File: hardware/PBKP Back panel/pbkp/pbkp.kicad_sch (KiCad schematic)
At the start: 9 parts, among them J1 Mini-DIN-6, J2 Mini-DIN-6, J3 RCA, J4 DB25_Male, J5 DB25_Female, J5 DB9_Male, J6 DB9_Female, J7 DB25_Female, J8 DB9_Female

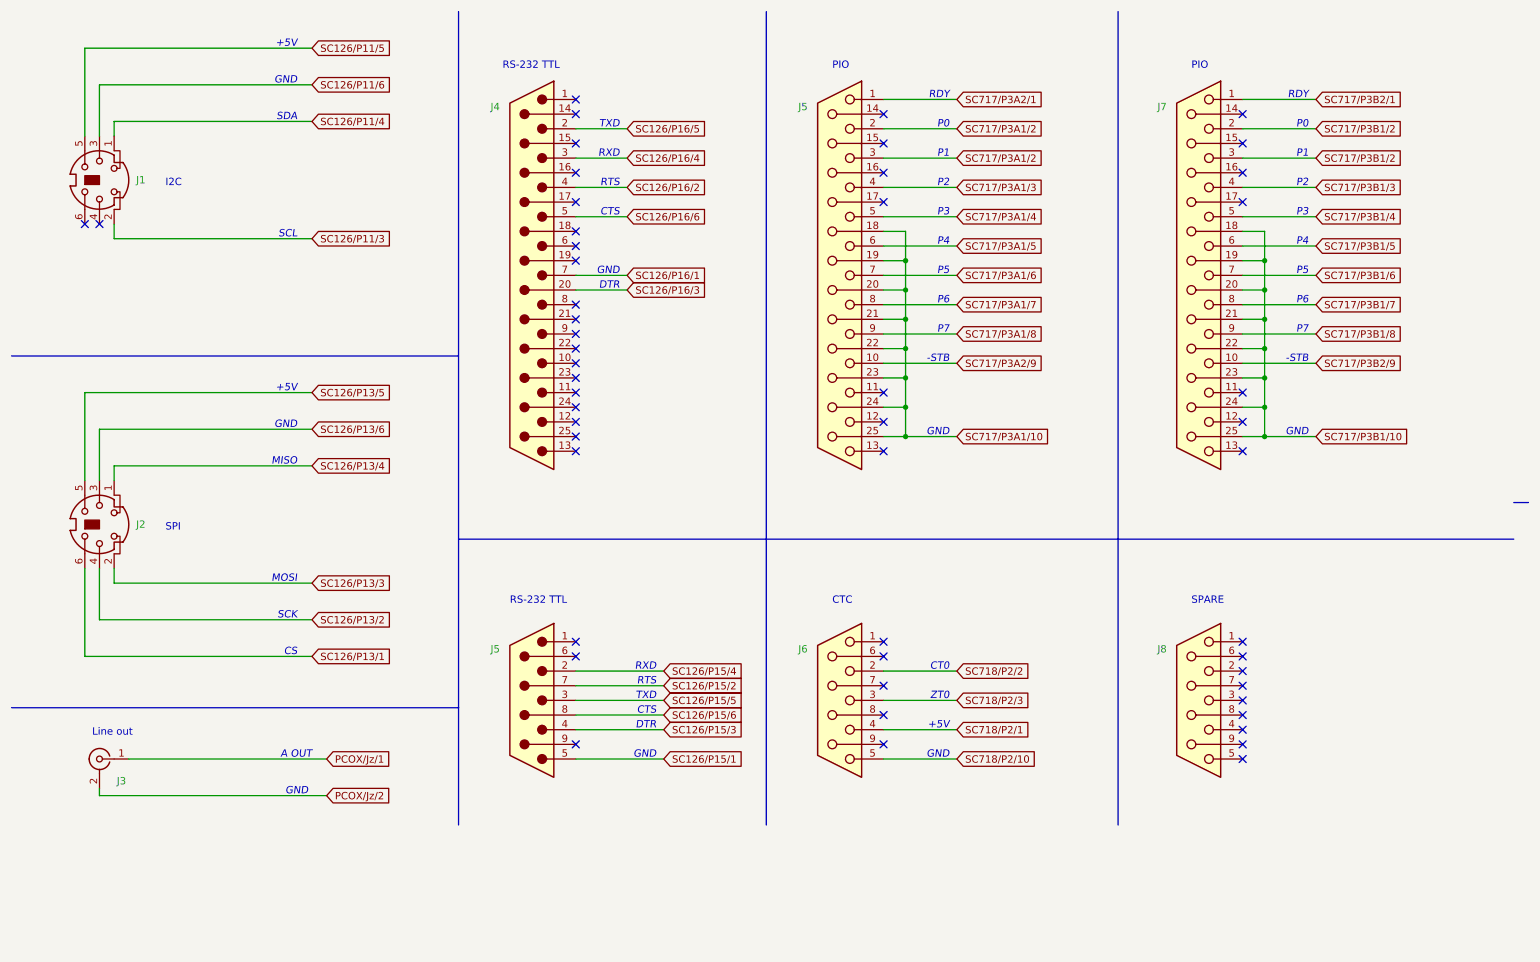
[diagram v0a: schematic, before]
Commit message: 251205
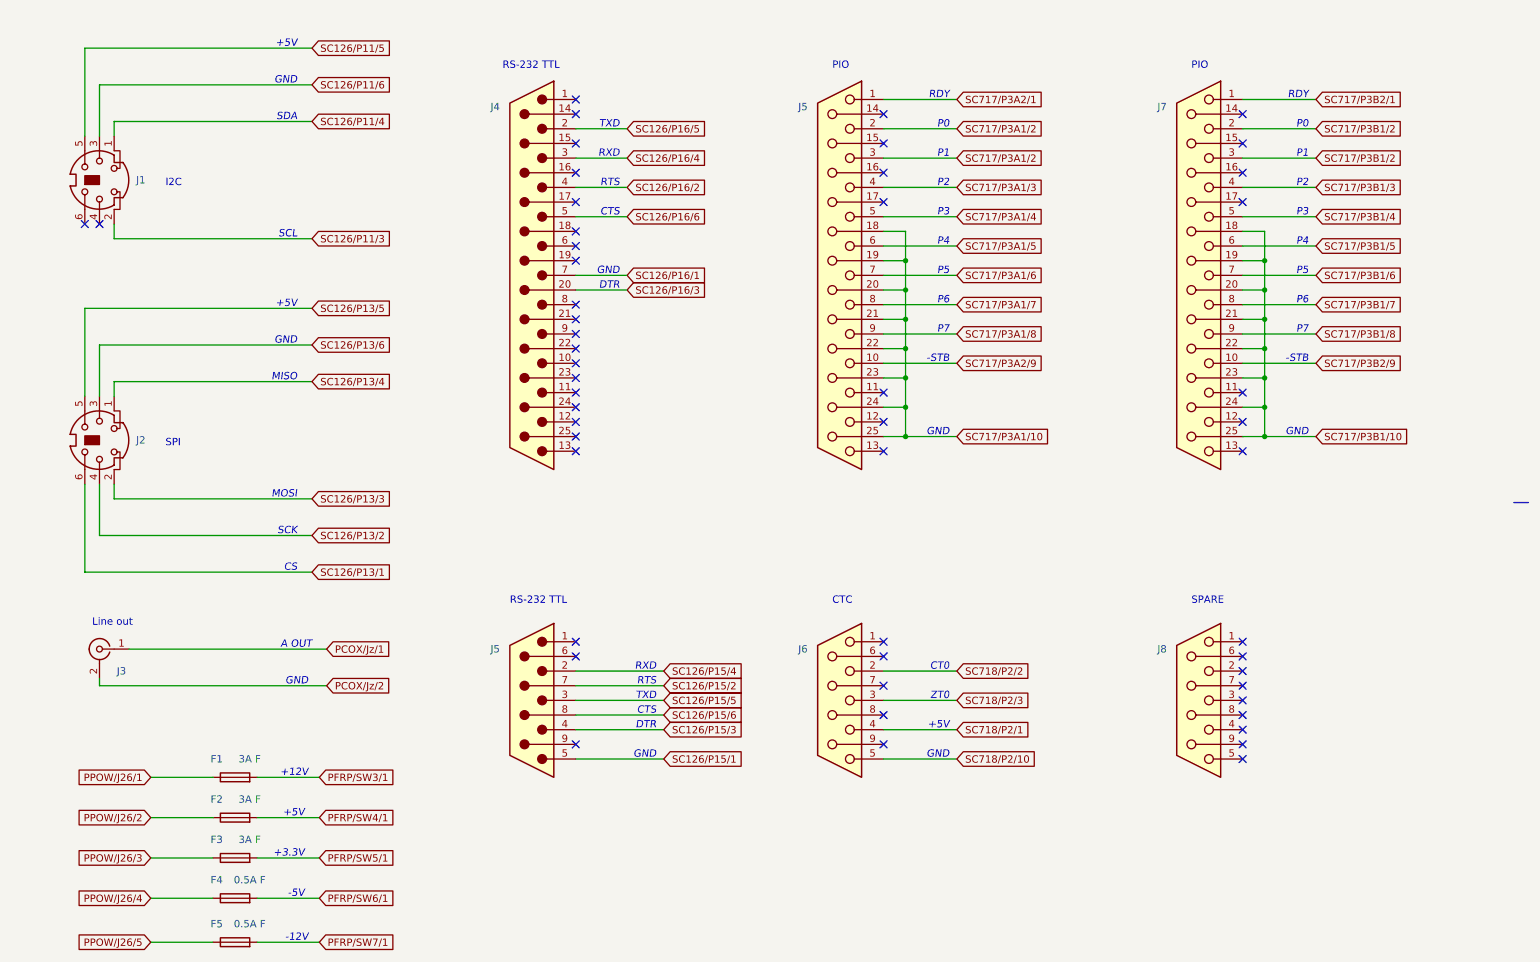
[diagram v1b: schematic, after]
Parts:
- added F1, F2, F3: 3A F, symbol Device:Fuse
- added F4, F5: 0.5A F, symbol Device:Fuse
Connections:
- new net PFRP/SW3/1: F1.2
- new net PFRP/SW4/1: F2.2
- new net PFRP/SW5/1: F3.2
- new net PFRP/SW6/1: F4.2
- new net PFRP/SW7/1: F5.2
- new net PPOW/J26/1: F1.1
- new net PPOW/J26/2: F2.1
- new net PPOW/J26/3: F3.1
- new net PPOW/J26/4: F4.1
- new net PPOW/J26/5: F5.1
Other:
- note added: "+12V"
- note added: "+3.3V"
- note added: "-12V"
- note added: "-5V"
- moved on the sheet: J2, J3
